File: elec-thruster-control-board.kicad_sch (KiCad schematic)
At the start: 45 parts, among them J1 Conn_01x20_Socket, J10 Conn_01x02_Socket, J11 Conn_01x02_Socket, J13 Conn_02x05_Counter_Clockwise, J14 Conn_01x02_Socket, J2 Conn_01x02_Socket, J3 Conn_01x20_Socket, J4 Conn_01x02_Socket, J5 Conn_01x02_Socket, J6 Conn_01x02_Socket, J7 Conn_01x02_Socket, J8 Conn_01x02_Socket, J9 Conn_01x02_Socket

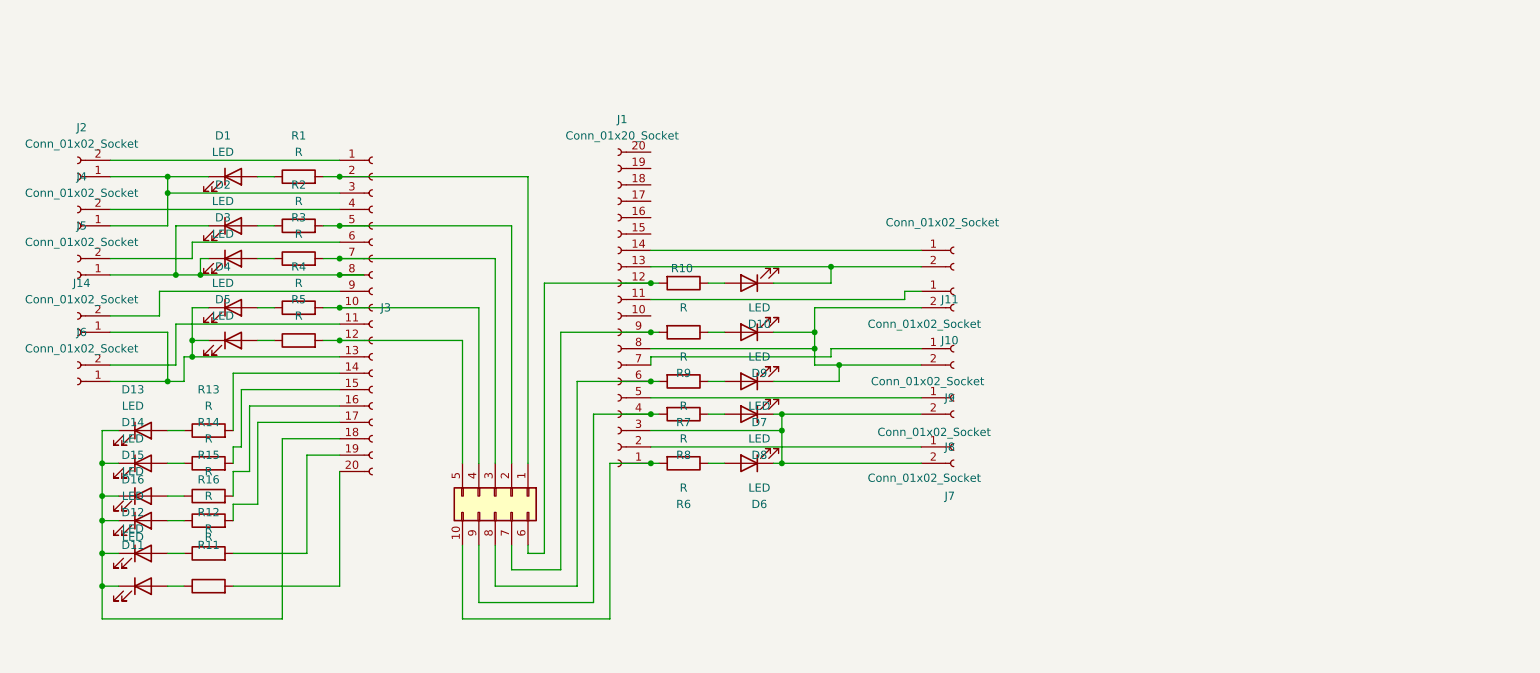
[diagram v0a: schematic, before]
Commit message: Update 4:25 rewired to fit a pico footprint
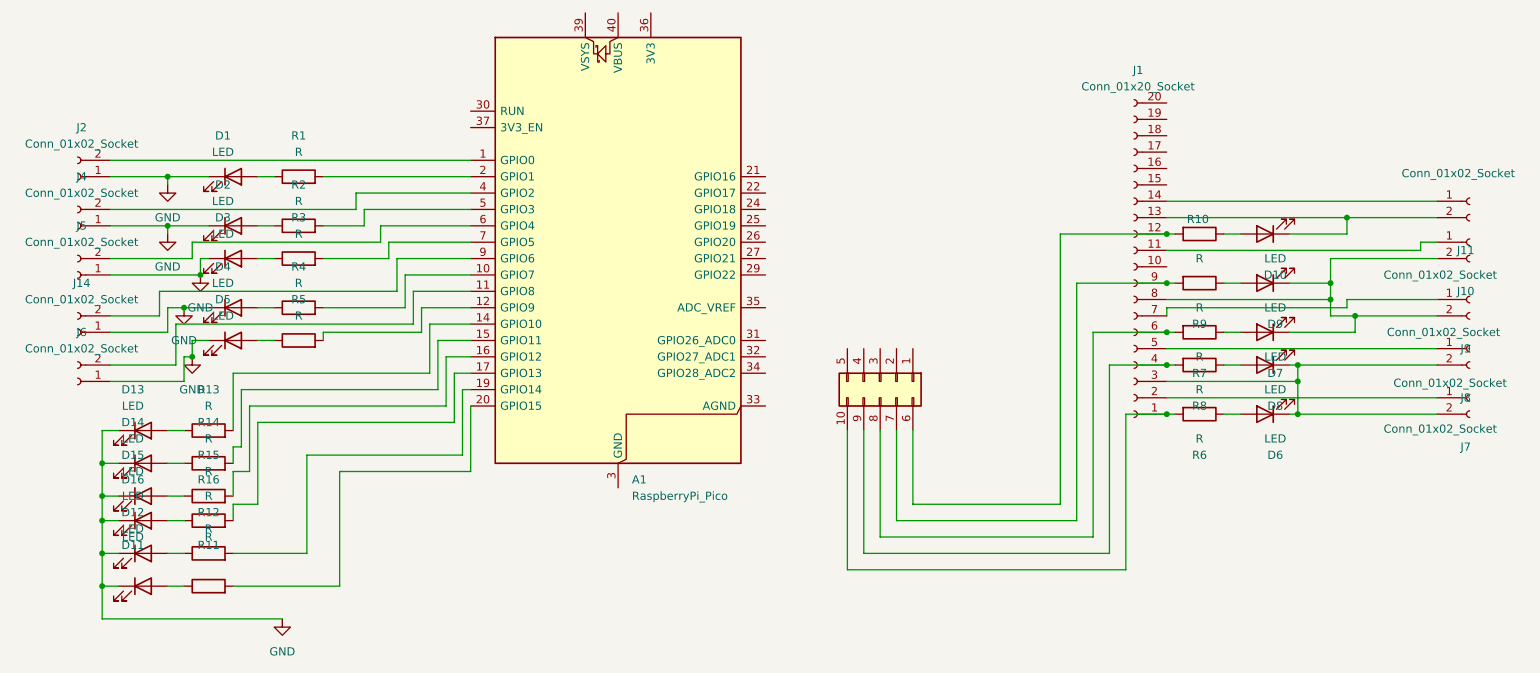
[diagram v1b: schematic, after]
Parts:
- removed J3: Conn_01x20_Socket, Connector_PinHeader_2.54mm:PinHeader_1x20_P2.54mm_Vertical_SMD_Pin1Left, symbol Connector:Conn_01x20_Socket
- added A1: RaspberryPi_Pico, Module:RaspberryPi_Pico_Common_THT, symbol MCU_Module:RaspberryPi_Pico
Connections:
- net GND: now reaches D1.1 (K), J2.1 (Pin_1), J4.1 (Pin_1)
- net GND: now also D11.1 (K), D12.1 (K), D13.1 (K), D14.1 (K), D15.1 (K), D16.1 (K), D2.1 (K), D3.1 (K), D4.1 (K), D5.1 (K), J14.1 (Pin_1), J5.1 (Pin_1), J6.1 (Pin_1)
- net at J4.2 (Pin_2): now also A1.4 (GPIO2)
- net at R16.2: now also A1.17 (GPIO13)
- net at R15.2: now also A1.16 (GPIO12)
- net at J2.2 (Pin_2): now also A1.1 (GPIO0)
- net at R3.2: now also A1.7 (GPIO5); no longer J13.3 (Pin_3)
- net at R1.2: now also A1.2 (GPIO1); no longer J13.1 (Pin_1)
- net at R2.2: now also A1.5 (GPIO3); no longer J13.2 (Pin_2)
- net at R4.2: now also A1.10 (GPIO7); no longer J13.4 (Pin_4)
- net at R5.2: now also A1.12 (GPIO9); no longer J13.5 (Pin_5)
- net at J6.2 (Pin_2): now also A1.11 (GPIO8)
- net at R13.2: now also A1.14 (GPIO10)
- net at R14.2: now also A1.15 (GPIO11)
- net at R12.2: now also A1.19 (GPIO14)
- net at R11.2: now also A1.20 (GPIO15)
- net at J5.2 (Pin_2): now also A1.6 (GPIO4)
- net at J14.2 (Pin_2): now also A1.9 (GPIO6)
- new net: A1.13 (GND), A1.18 (GND), A1.23 (GND), A1.28 (GND), A1.3 (GND), A1.38 (GND), A1.8 (GND)
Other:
- moved on the sheet: D10, D6, D7, D8, D9, J1, J10, J11, J7, J8, J9, R10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
